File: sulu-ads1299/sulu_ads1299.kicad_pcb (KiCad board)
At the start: 2 copper layers, 35.8 x 42.8 mm, 78 parts, among them J1 Conn_01x08, J11 through_hole, J16 through_hole, J2 Conn_01x02, J20 through_hole, J3 Conn_02x05_Odd_Even, J4 through_hole, J5 through_hole, J6 through_hole, J7 Conn_01x08, J8 through_hole, Q1 BSS138, Q2 BSS138, SW1 SW_DIP_x02, U1 TPS62222DDCT, U2 TPS62222DDCT, U3 LM2775DSG, U4 ADS1299_TQFP-64, U5 scum3

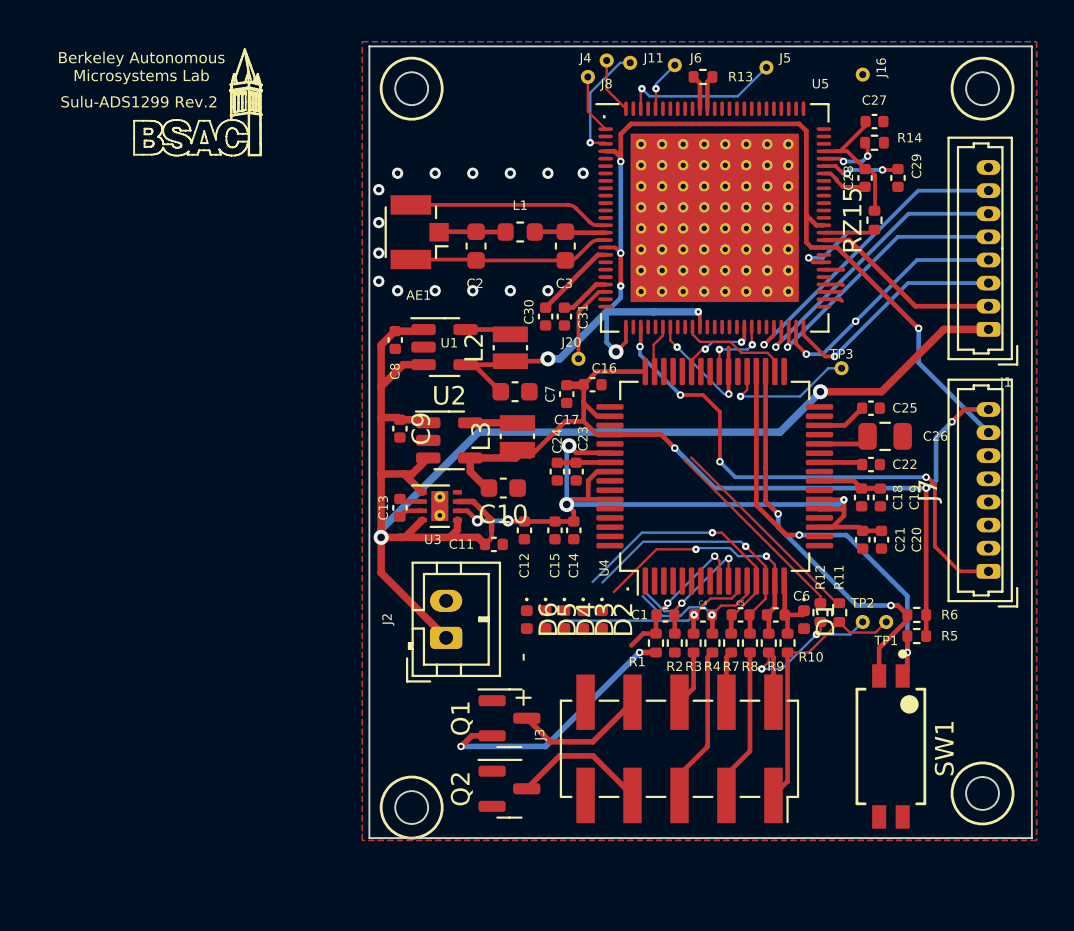
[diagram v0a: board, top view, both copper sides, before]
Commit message: DRC clean layout of Rev. 3
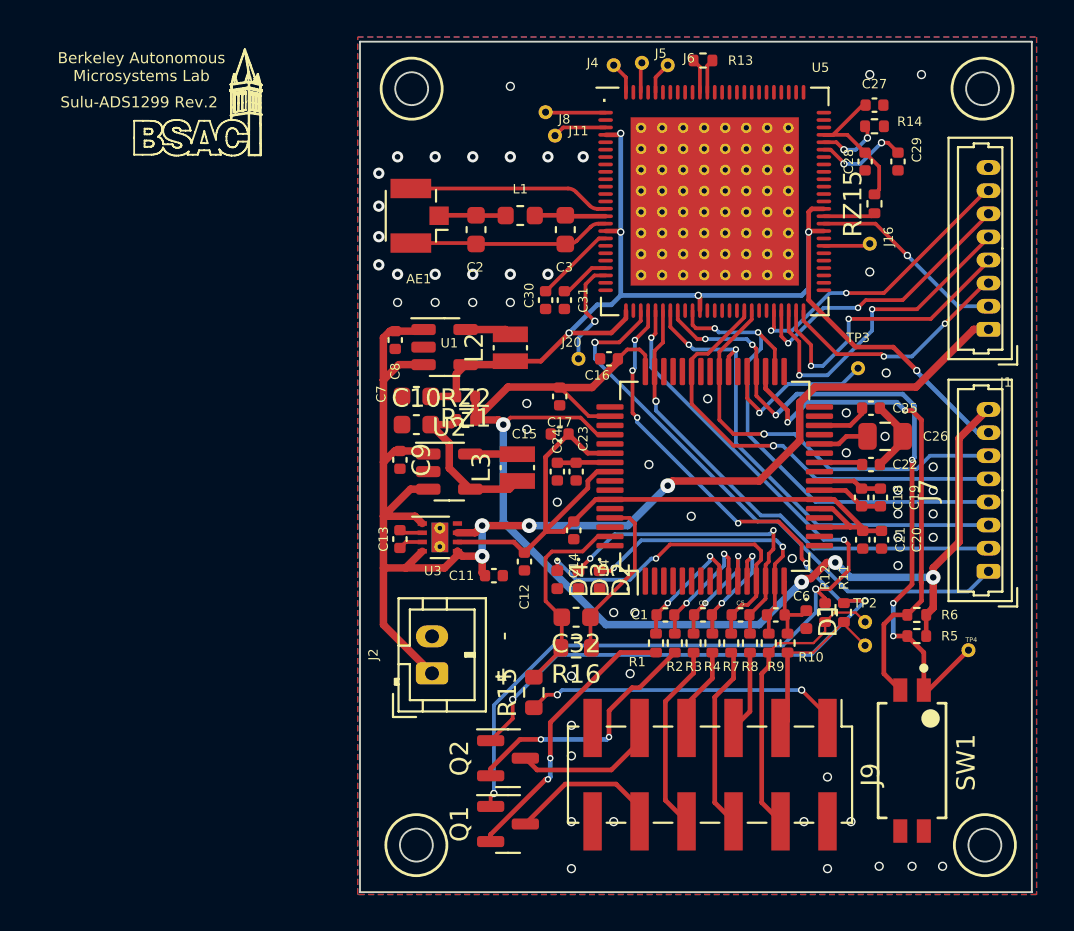
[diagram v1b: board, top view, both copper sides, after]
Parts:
- removed D5, D6: GDZ5V1LP3-7, Diode_SMD:D_0402_1005Metric
- removed J3: Conn_02x05_Odd_Even, Connector_PinSocket_2.54mm:PinSocket_2x05_P2.54mm_Vertical_SMD
- added C32: 0.01uF, Capacitor_SMD:C_0603_1608Metric, F.Cu at (96.1, 81.9)
- added J9: Conn_02x06_Odd_Even, Connector_PinHeader_2.54mm:PinHeader_2x06_P2.54mm_Vertical_SMD, F.Cu at (103.4, 90.4)
- added R15: 4.99K, Resistor_SMD:R_0603_1608Metric, F.Cu at (93.9, 86.0)
- added R16: 392K, Resistor_SMD:R_0603_1608Metric, F.Cu at (96.1, 83.6)
- added RZ1: 0 Ohm, Resistor_SMD:R_0402_1005Metric, F.Cu at (90.2, 70.0)
- added RZ2: NP, Resistor_SMD:R_0402_1005Metric, F.Cu at (90.2, 71.2)
- added TP4: TestPoint, SCUM:through_hole, F.Cu at (117.3, 83.7)
- TP1: moved to B.Cu
- moved J16 9.15 mm to (112.0, 61.7)
- moved J5 6.74 mm to (99.7, 51.9)
- moved C10 5.82 mm to (87.5, 71.5), turned to 0 degrees
- moved Q1 5.72 mm to (92.5, 93.1)
- moved J11 5.66 mm to (95.0, 55.9)
- moved C7 5.34 mm to (87.5, 70.0), turned to 0 degrees
- moved C15 5.21 mm to (95.2, 72.0), turned to 180 degrees
- moved J8 2.98 mm to (94.5, 54.6)
- moved D4 2.19 mm to (95.1, 79.9)
- moved D3 2.17 mm to (96.3, 79.9)
- moved D2 2.16 mm to (97.4, 79.9)
- moved J2 2.07 mm to (88.3, 84.9)
- moved TP1 1.71 mm to (111.8, 83.4), turned to 180 degrees
- moved C11 1.69 mm to (91.7, 79.7)
- moved C12 1.69 mm to (93.3, 78.9)
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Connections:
- C10 pad 2: /+1.8V_ADS -> /+1.8V_BACKUP
- L3 pad 1: /+1.8V_ADS -> /+1.8V_BACKUP
- U2 pad 4: /+1.8V_ADS -> /+1.8V_BACKUP
- U4 pad 61: unconnected-(U4-Pad61) -> /ADS1299/BIASINV
- U4 pad 63: unconnected-(U4-Pad63) -> /ADS1299/BIASOUT
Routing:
- net /SCUM_GPIO2: track 10.8 -> 48.7 mm, vias 0 -> 4
- net /SCUM_GPIO1: track 11.3 -> 48.6 mm, vias 0 -> 7
- net /SCUM_GPIO3: track 2.64 -> 26.7 mm, vias 0 -> 1
- net /SCUM_GPIO7: track 5.64 -> 27.4 mm, vias 0 -> 2
- net /SCUM_GPIO13: track 4.61 -> 24.3 mm, vias 2 -> 1
- net /SCUM_GPIO4: track 7.68 -> 26.9 mm
- net /+1.8V_ADS: track 51.8 -> 70.7 mm, vias 3 -> 4
- net /SCUM_GPIO14: track 4.05 -> 22.6 mm, vias 2 -> 1
- net /ADS_BIAS_ELEC: track 0.00 -> 17.5 mm, vias 0 -> 2
- net /SCUM_GPIO5: track 22.7 -> 37.9 mm, vias 2 -> 6
- net Net-(Q2-Pad2): track 0.00 -> 13.8 mm, vias 0 -> 2
- net /ADS1299/BIASOUT: track 0.00 -> 11.4 mm
- net /ADS1299/BIASINV: track 0.00 -> 9.21 mm
- net /+1.8V_BACKUP: track 0.00 -> 8.59 mm
- net /ADS_IN3N_CONN: track 3.00 -> 10.2 mm
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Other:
- board size 35.8 x 42.8 mm -> 36.3 x 46 mm
